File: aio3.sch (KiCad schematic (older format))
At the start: 24 parts, among them SW1 SW_Push, U1 ATmega32U4-AU, Y1 16MHz

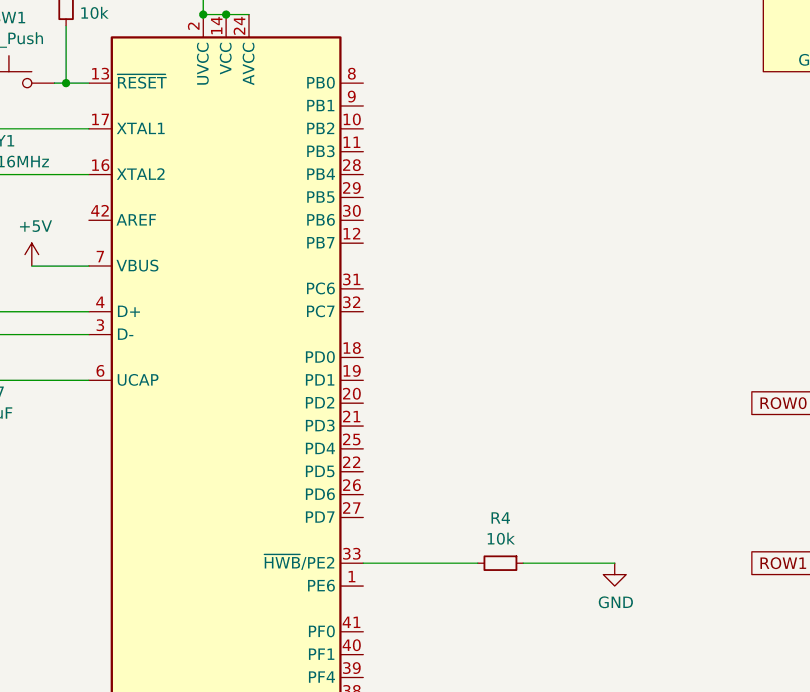
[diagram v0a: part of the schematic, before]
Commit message: Finished Board. Maybe.
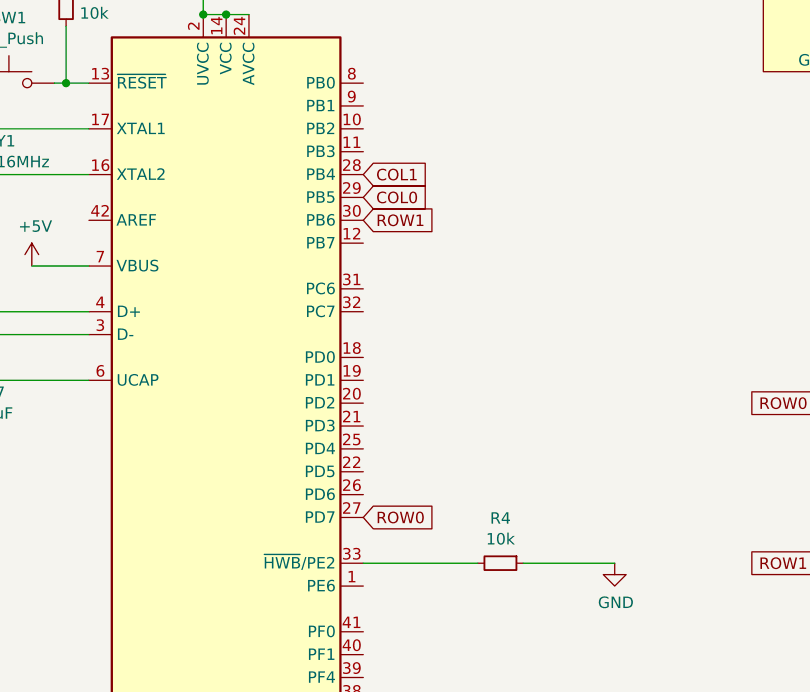
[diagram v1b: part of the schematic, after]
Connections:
- net COL0: now also U1.29 (PB5)
- net COL1: now also U1.28 (PB4)
- net ROW0: now also U1.27 (PD7)
- net ROW1: now also U1.30 (PB6)
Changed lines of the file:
@@
 Text GLabel 8400 4150 0    50   Input ~ 0
 ROW1
+Text GLabel 6400 2450 2    50   Input ~ 0
+COL1
+Text GLabel 6400 2550 2    50   Input ~ 0
+COL0
+Text GLabel 6400 2650 2    50   Input ~ 0
+ROW1
+Text GLabel 6400 3950 2    50   Input ~ 0
+ROW0
 $EndSCHEMATC
